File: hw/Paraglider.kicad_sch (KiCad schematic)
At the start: 8 parts, among them J1 Raspberry_Pi_4, J2 Conn GPS, J3 Load Cell, J4 Conn_01x08_MountingPin, U1 HX711, U4 CP2102N-Axx-xQFN20

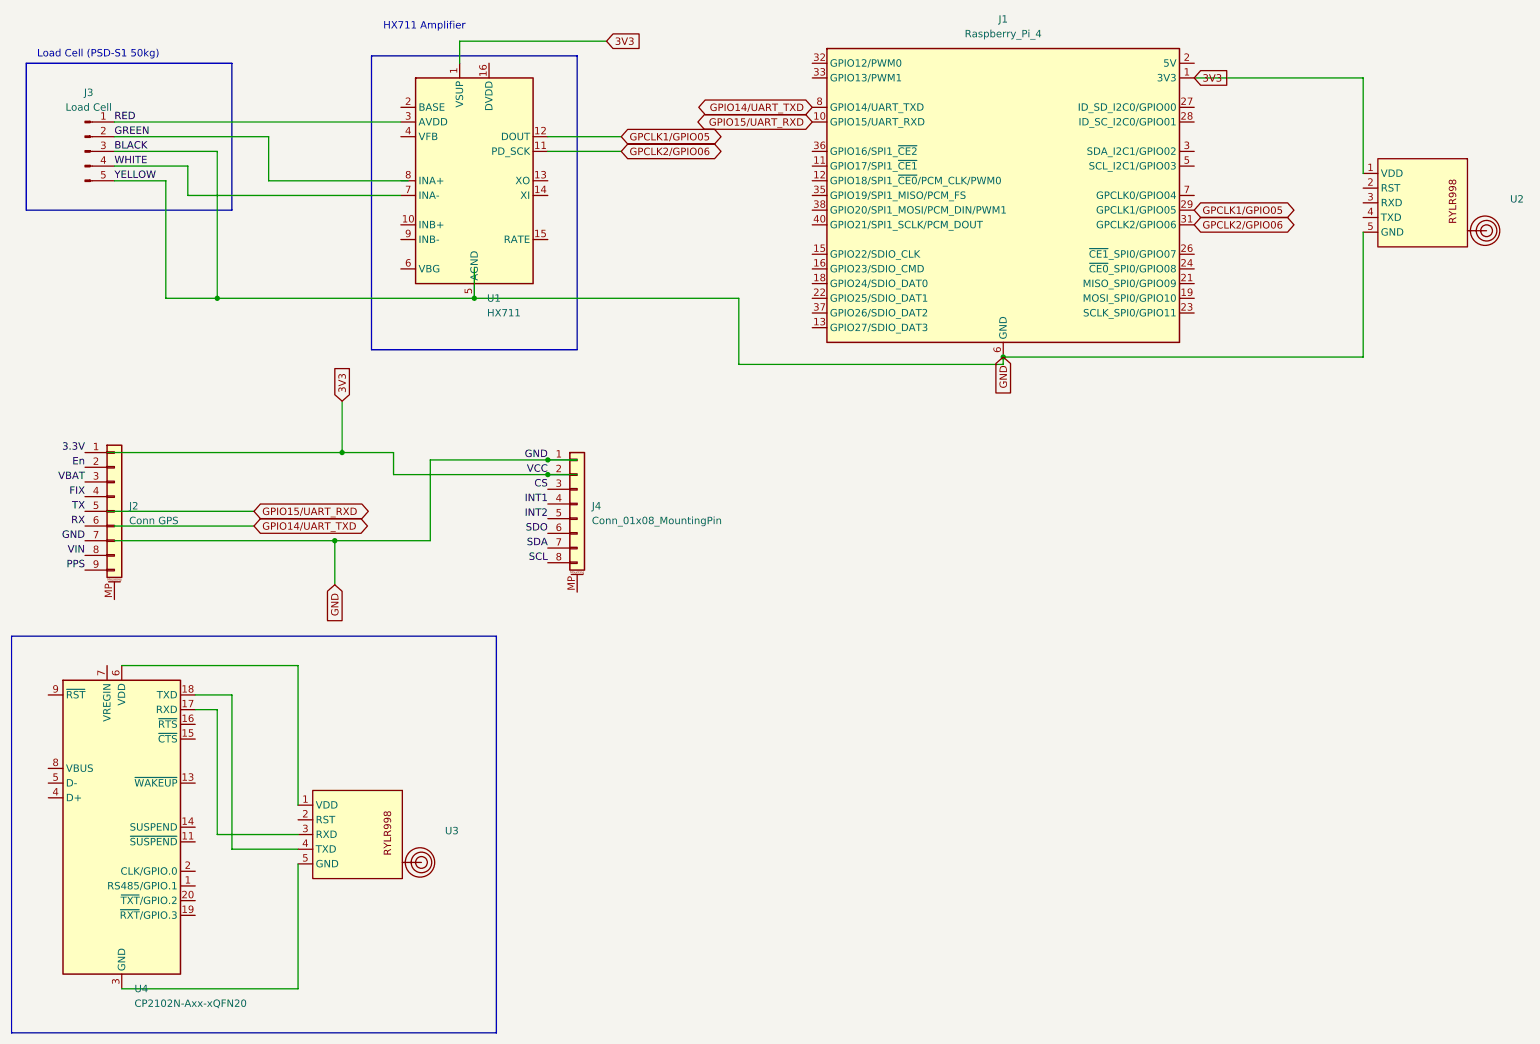
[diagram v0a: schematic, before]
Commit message: kicad hw
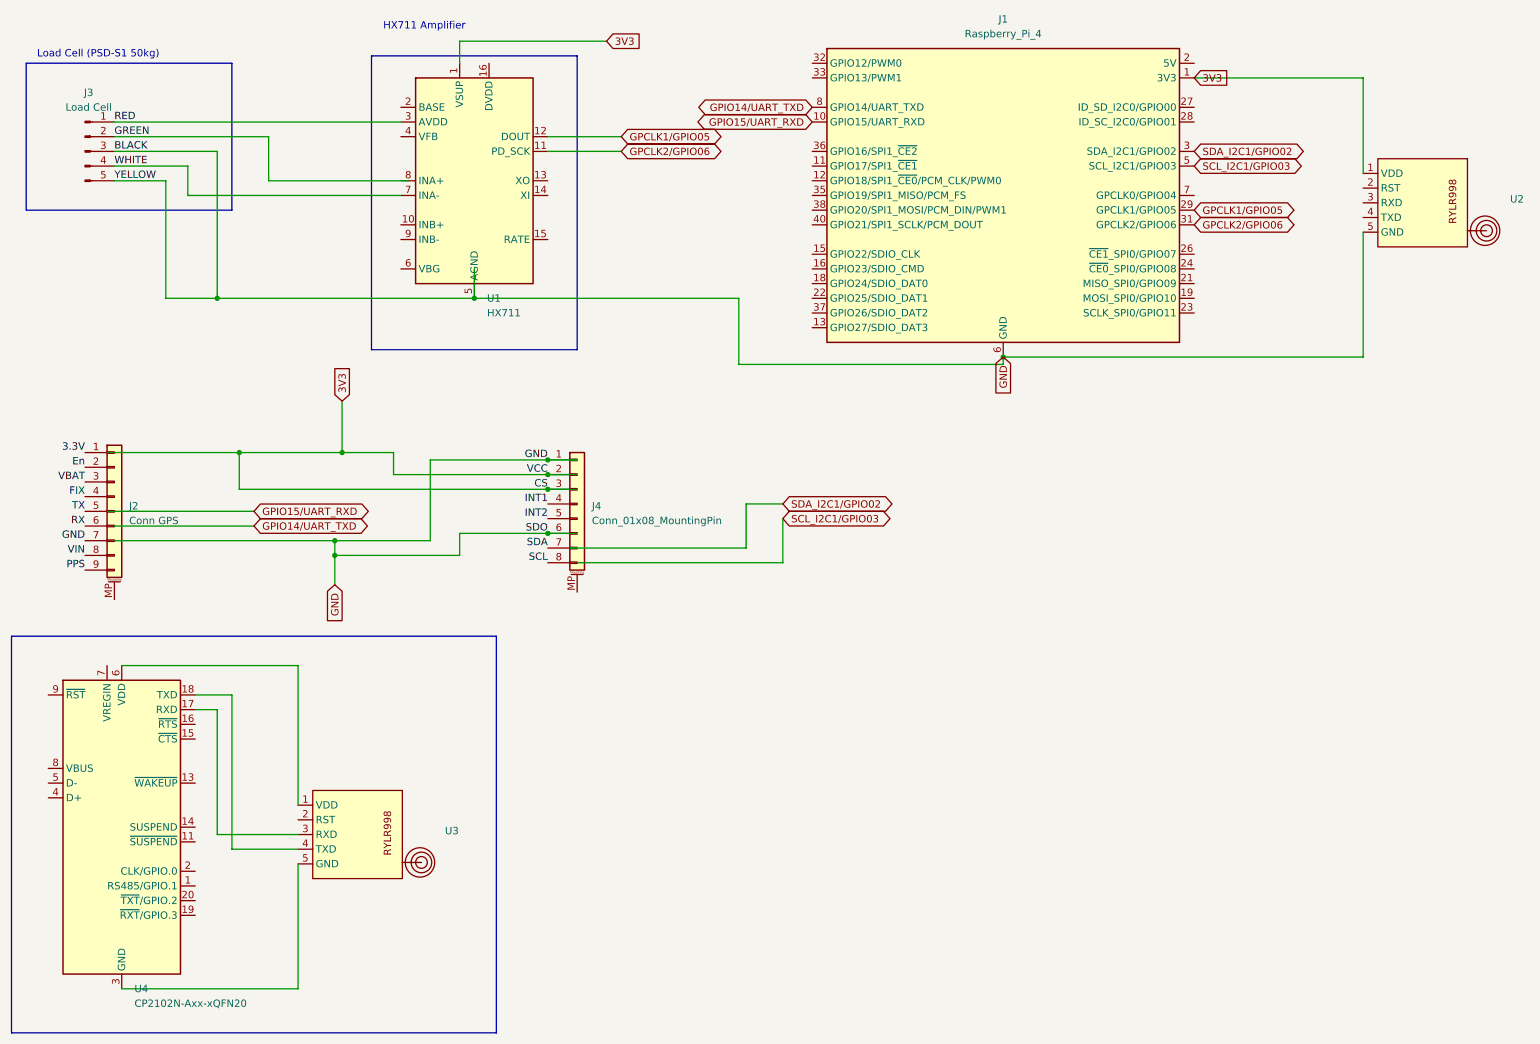
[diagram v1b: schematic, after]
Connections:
- net CS is gone; now on net 3V3: J4.3 (Pin_3)
- net SDO is gone; now on net GND: J4.6 (Pin_6)
- net SDA_I2C1/GPIO02: now reaches J1.3 (SDA_I2C1/GPIO02)
- net SCL_I2C1/GPIO03: now reaches J1.5 (SCL_I2C1/GPIO03)
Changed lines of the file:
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@@
+	)
+	(junction
+		(at 113.03 109.22)
+		(diameter 0)
+		(color 0 0 0 0)
 	)
 	(junction
@@
 	)
 	(junction
+		(at 59.69 95.25)
+		(diameter 0)
+		(color 0 0 0 0)
+	)
+	(junction
 		(at 77.47 95.25)
 		(diameter 0)
@@
 		(color 0 0 0 0)
 	)
+	(junction
+		(at 113.03 101.6)
+		(diameter 0)
+		(color 0 0 0 0)
+	)
+	(junction
+		(at 76.2 113.03)
+		(diameter 0)
+		(color 0 0 0 0)
+	)
 	(wire
 		(pts
@@
 	(wire
 		(pts
+			(xy 59.69 101.6) (xy 59.69 95.25)
+		)
+		(stroke
+			(width 0)
+			(type default)
+		)
+	)
+	(wire
+		(pts
 			(xy 58.42 137.16) (xy 58.42 163.83)
 		)
@@
 	(wire
 		(pts
+			(xy 59.69 95.25) (xy 36.83 95.25)
+		)
+		(stroke
+			(width 0)
+			(type default)
+		)
+	)
+	(wire
+		(pts
 			(xy 146.05 80.01) (xy 191.77 80.01)
 		)
@@
 	(wire
 		(pts
+			(xy 113.03 101.6) (xy 118.11 101.6)
+		)
+		(stroke
+			(width 0)
+			(type default)
+		)
+	)
+	(wire
+		(pts
 			(xy 86.36 99.06) (xy 86.36 95.25)
 		)
@@
 	(wire
 		(pts
+			(xy 116.84 111.76) (xy 147.32 111.76)
+		)
+		(stroke
+			(width 0)
+			(type default)
+		)
+	)
+	(wire
+		(pts
 			(xy 113.03 99.06) (xy 86.36 99.06)
 		)
@@
 	(wire
 		(pts
+			(xy 97.79 109.22) (xy 97.79 113.03)
+		)
+		(stroke
+			(width 0)
+			(type default)
+		)
+	)
+	(wire
+		(pts
 			(xy 55.88 139.7) (xy 52.07 139.7)
 		)
@@
 	(wire
 		(pts
+			(xy 147.32 111.76) (xy 147.32 104.14)
+		)
+		(stroke
+			(width 0)
+			(type default)
+		)
+	)
+	(wire
+		(pts
 			(xy 69.85 132.08) (xy 39.37 132.08)
 		)
@@
 	(wire
 		(pts
+			(xy 76.2 113.03) (xy 76.2 110.49)
+		)
+		(stroke
+			(width 0)
+			(type default)
+		)
+	)
+	(wire
+		(pts
 			(xy 92.71 110.49) (xy 76.2 110.49)
 		)
@@
 	(wire
 		(pts
+			(xy 59.69 101.6) (xy 113.03 101.6)
+		)
+		(stroke
+			(width 0)
+			(type default)
+		)
+	)
+	(wire
+		(pts
 			(xy 123.19 24.13) (xy 97.79 24.13)
 		)
@@
 	(wire
 		(pts
+			(xy 113.03 109.22) (xy 97.79 109.22)
+		)
+		(stroke
+			(width 0)
+			(type default)
+		)
+	)
+	(wire
+		(pts
 			(xy 69.85 187.96) (xy 69.85 166.37)
 		)
@@
 	(wire
 		(pts
+			(xy 118.11 109.22) (xy 113.03 109.22)
+		)
+		(stroke
+			(width 0)
+			(type default)
+		)
+	)
+	(wire
+		(pts
 			(xy 69.85 156.21) (xy 69.85 132.08)
 		)
@@
 	(wire
 		(pts
-			(xy 76.2 118.11) (xy 76.2 110.49)
+			(xy 76.2 118.11) (xy 76.2 113.03)
+		)
+		(stroke
+			(width 0)
+			(type default)
+		)
+	)
+	(wire
+		(pts
+			(xy 97.79 113.03) (xy 76.2 113.03)
 		)
 		(stroke
@@
 	(wire
 		(pts
+			(xy 118.11 114.3) (xy 153.67 114.3)
+		)
+		(stroke
+			(width 0)
+			(type default)
+		)
+	)
+	(wire
+		(pts
+			(xy 147.32 104.14) (xy 153.67 104.14)
+		)
+		(stroke
+			(width 0)
+			(type default)
+		)
+	)
+	(wire
+		(pts
 			(xy 46.99 48.26) (xy 46.99 68.58)
 		)
@@
 	(wire
 		(pts
-			(xy 77.47 95.25) (xy 36.83 95.25)
+			(xy 59.69 95.25) (xy 77.47 95.25)
 		)
 		(stroke
@@
 		(pts
 			(xy 58.42 163.83) (xy 69.85 163.83)
+		)
+		(stroke
+			(width 0)
+			(type default)
+		)
+	)
+	(wire
+		(pts
+			(xy 153.67 114.3) (xy 153.67 106.68)
 		)
 		(stroke
@@
 		)
 	)
+	(global_label "SDA_I2C1/GPIO02"
+		(shape bidirectional)
+		(at 224.79 43.18 0)
+		(effects
+			(font
+				(size 1.27 1.27)
+			)
+			(justify left)
+		)
+		(property "Intersheetrefs" "${INTERSHEET_REFS}"
+			(at 224.79 43.18 0)
+			(effects
+				(font
+					(size 1.27 1.27)
+				)
+				(hide yes)
+			)
+		)
+	)
 	(global_label "3V3"
 		(shape input)
@@
 		)
 	)
+	(global_label "SCL_I2C1/GPIO03"
+		(shape bidirectional)
+		(at 224.79 45.72 0)
+		(effects
+			(font
+				(size 1.27 1.27)
+			)
+			(justify left)
+		)
+		(property "Intersheetrefs" "${INTERSHEET_REFS}"
+			(at 224.79 45.72 0)
+			(effects
+				(font
+					(size 1.27 1.27)
+				)
+				(hide yes)
+			)
+		)
+	)
+	(global_label "SDA_I2C1/GPIO02"
+		(shape bidirectional)
+		(at 153.67 104.14 0)
+		(effects
+			(font
+				(size 1.27 1.27)
+			)
+			(justify left)
+		)
+		(property "Intersheetrefs" "${INTERSHEET_REFS}"
+			(at 153.67 104.14 0)
+			(effects
+				(font
+					(size 1.27 1.27)
+				)
+				(hide yes)
+			)
+		)
+	)
 	(global_label "GPIO14/UART_TXD"
 		(shape bidirectional)
@@
 			(effects
 				(font
+					(size 1.27 1.27)
+				)
+				(hide yes)
+			)
+		)
+	)
+	(global_label "SCL_I2C1/GPIO03"
+		(shape bidirectional)
+		(at 153.67 106.68 0)
+		(effects
+			(font
+				(size 1.27 1.27)
+			)
+			(justify left)
+		)
+		(property "Intersheetrefs" "${INTERSHEET_REFS}"
+			(at 153.67 106.68 0)
+			(effects
+				(font

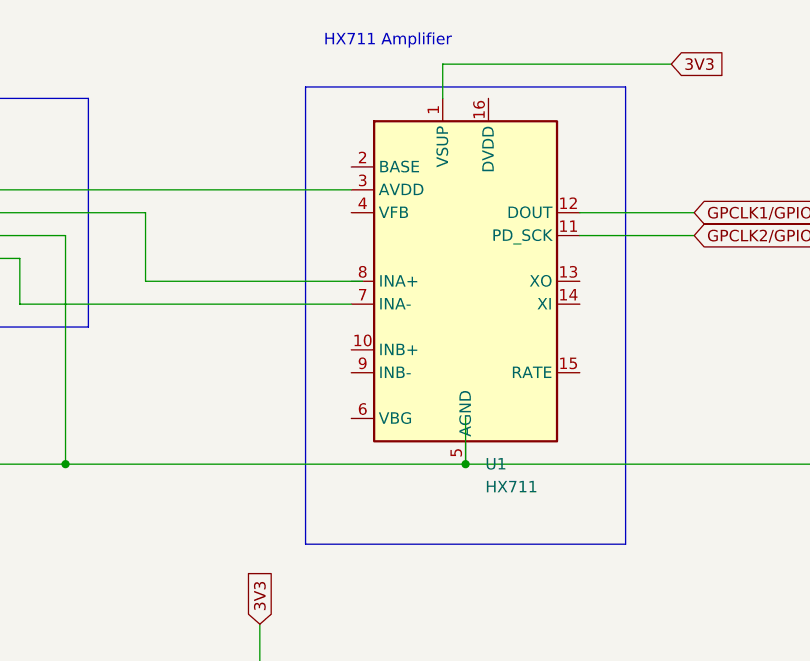
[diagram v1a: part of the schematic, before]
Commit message: movement
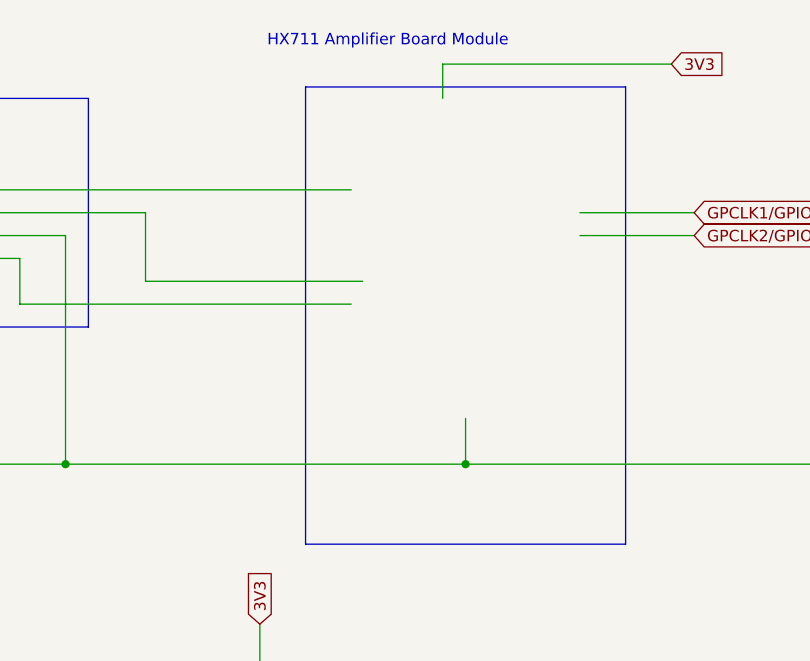
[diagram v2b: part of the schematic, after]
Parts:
- removed U1: HX711, Package_SO:SOP-16_3.9x9.9mm_P1.27mm, symbol Analog_ADC:HX711
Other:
- note added: "HX711 Amplifier Board Module"
- note removed: "HX711 Amplifier"
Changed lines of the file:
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@@
 		)
 	)
-	(text "HX711 Amplifier"
+	(text "HX711 Amplifier Board Module"
 		(exclude_from_sim no)
 		(at 91.694 21.59 0)
@@
 					(unit 1)
 				)
-			)
-		)
-	)
-	(symbol
-		(lib_id "Analog_ADC:HX711")
-		(at 100.33 48.26 0)
-		(unit 1)
-		(exclude_from_sim no)
-		(in_bom yes)
-		(on_board yes)
-		(dnp no)
-		(fields_autoplaced yes)
-		(property "Reference" "U1"
-			(at 102.5241 68.58 0)
-			(effects
-				(font
-					(size 1.27 1.27)
-				)
-				(justify left)
-			)
-		)
-		(property "Value" "HX711"
-			(at 102.5241 71.12 0)
-			(effects
-				(font
-					(size 1.27 1.27)
-				)
-				(justify left)
-			)
-		)
-		(property "Footprint" "Package_SO:SOP-16_3.9x9.9mm_P1.27mm"
-			(at 104.14 46.99 0)
-			(effects
-				(font
-					(size 1.27 1.27)
-				)
-				(hide yes)
-			)
-		)
-		(property "Datasheet" "https://web.archive.org/web/20220615044707/https://akizukidenshi.com/download/ds/avia/hx711.pdf"
-			(at 104.14 49.53 0)
-			(effects
-				(font
-					(size 1.27 1.27)
-				)
-				(hide yes)
-			)
-		)
-		(property "Description" "24-Bit Analog-to-Digital Converter (ADC) for Weight Scales"
-			(at 100.33 48.26 0)
-			(effects
-				(font
-					(size 1.27 1.27)
-				)
-				(hide yes)
-			)
-		)
-		(pin "13"
-		)
-		(pin "14"
-		)
-		(pin "1"
-		)
-		(pin "10"
-		)
-		(pin "2"
-		)
-		(pin "6"
-		)
-		(pin "4"
-		)
-		(pin "16"
-		)
-		(pin "15"
-		)
-		(pin "5"
-		)
-		(pin "8"
-		)
-		(pin "11"
-		)
-		(pin "3"
-		)
-		(pin "12"
-		)
-		(pin "7"
-		)
-		(pin "9"
-		)
-		(instances
-			(project ""
-				(path "/51c9047f-980c-4c4c-b786-6f97d4faa6b2"
-					(reference "U1")
-					(unit 1)
-				)
